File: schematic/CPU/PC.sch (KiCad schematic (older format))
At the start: 9 parts, among them U52 74LS86, U53 74LS08, U54 74LS86, U55 74LS08, U56 74LS273, U57 74LS157, U58 74LS157, U59 74LS32, U60 74LS245

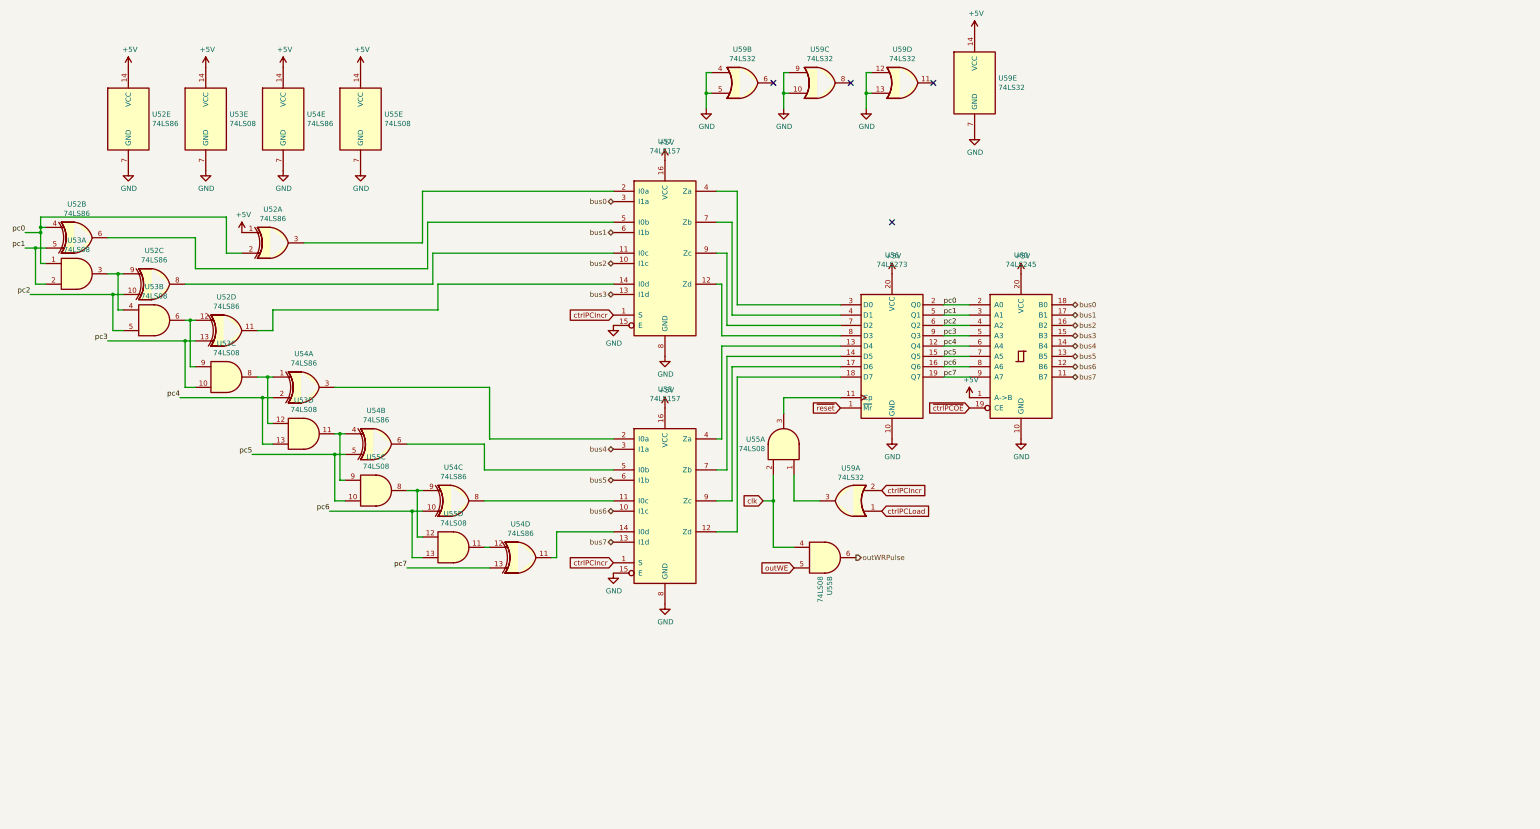
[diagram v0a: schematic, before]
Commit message: schematic finished
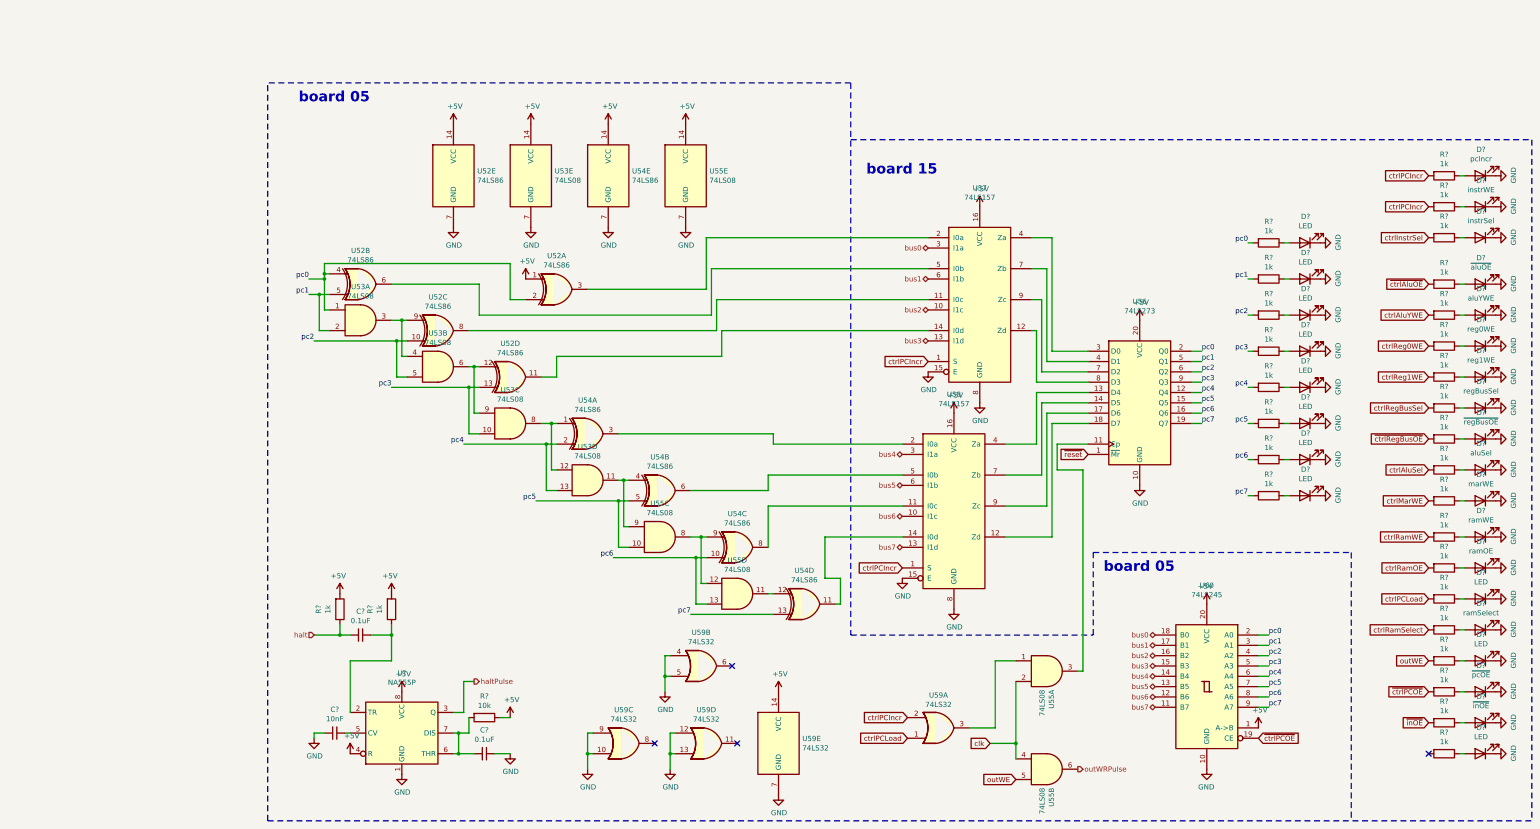
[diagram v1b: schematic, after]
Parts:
- added C? (x2): 0.1uF, symbol Device:C_Small
- added C?: 10nF, symbol Device:C_Small
- added D?: ~regBusOE~, LED_THT:LED_D3.0mm, symbol Device:LED
- added D?: aluSel, LED_THT:LED_D3.0mm, symbol Device:LED
- added D?: marWE, LED_THT:LED_D3.0mm, symbol Device:LED
- added D?: ramWE, LED_THT:LED_D3.0mm, symbol Device:LED
- added D?: ramOE, LED_THT:LED_D3.0mm, symbol Device:LED
- added D? (x11): LED, LED_THT:LED_D3.0mm, symbol Device:LED
- added D?: ramSelect, LED_THT:LED_D3.0mm, symbol Device:LED
- added D?: regBusSel, LED_THT:LED_D3.0mm, symbol Device:LED
- added D?: reg1WE, LED_THT:LED_D3.0mm, symbol Device:LED
- added D?: reg0WE, LED_THT:LED_D3.0mm, symbol Device:LED
- added D?: aluYWE, LED_THT:LED_D3.0mm, symbol Device:LED
- added D?: ~aluOE~, LED_THT:LED_D3.0mm, symbol Device:LED
- added D?: ~pcOE~, LED_THT:LED_D3.0mm, symbol Device:LED
- added D?: ~inOE~, LED_THT:LED_D3.0mm, symbol Device:LED
- added D?: instrSel, LED_THT:LED_D3.0mm, symbol Device:LED
- added D?: instrWE, LED_THT:LED_D3.0mm, symbol Device:LED
- added D?: pcIncr, LED_THT:LED_D3.0mm, symbol Device:LED
- added R? (x29): 1k, Resistor_THT:R_Axial_DIN0207_L6.3mm_D2.5mm_P7.62mm_Horizontal, symbol Device:R
- added R?: 10k, Resistor_THT:R_Axial_DIN0207_L6.3mm_D2.5mm_P7.62mm_Horizontal, symbol Device:R
- added U?: NA555P, Package_DIP:DIP-8_W7.62mm, symbol Timer:NA555P
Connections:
- net +5V: now also R?.1, R?.2, R?.2, U?.4 (R), U?.8 (VCC)
- net GND: now also C?.1, C?.2, D?.1 (K), D?.1 (K), D?.1 (K), D?.1 (K), D?.1 (K), D?.1 (K), D?.1 (K), D?.1 (K), D?.1 (K), D?.1 (K), D?.1 (K), D?.1 (K), D?.1 (K), D?.1 (K), D?.1 (K), D?.1 (K), D?.1 (K), D?.1 (K), D?.1 (K), D?.1 (K), D?.1 (K), D?.1 (K), D?.1 (K), D?.1 (K), D?.1 (K), D?.1 (K), D?.1 (K), U?.1 (GND)
- net ctrlPCIncr: now also R?.2, R?.2
- net ctrlPCLoad: now also R?.2
- net outWE: now also R?.2
- net pc0: now also R?.2
- net pc1: now also R?.2
- net pc2: now also R?.2
- net pc3: now also R?.2
- net pc4: now also R?.2
- net pc5: now also R?.2
- net pc6: now also R?.2
- net pc7: now also R?.2
- net ~ctrlPCOE~: now also R?.2
- new net: C?.2, R?.1, U?.2 (TR)
- new net: C?.1, U?.5 (CV)
- new net: C?.2, R?.2, U?.6 (THR), U?.7 (DIS)
- new net: D?.2 (A), R?.1 (x27)
- new net ctrlAluSel: R?.2
- new net ctrlAluYWE: R?.2
- new net ctrlInstrSel: R?.2
- new net ctrlMarWE: R?.2
- new net ctrlRamOE: R?.2
- new net ctrlRamSelect: R?.2
- new net ctrlRamWE: R?.2
- new net ctrlReg0WE: R?.2
- new net ctrlReg1WE: R?.2
- new net ctrlRegBusSel: R?.2
- new net halt: C?.1, R?.1
- new net haltPulse: U?.3 (Q)
- new net ~ctrlAluOE~: R?.2
- new net ~ctrlRegBusOE~: R?.2
- new net ~inOE~: R?.2
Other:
- note added: "board 05"
- note added: "board 15"
- moved on the sheet: U52A, U52B, U52C, U52D, U52E, U53A, U53B, U53C, U53D, U53E, U54A, U54B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
